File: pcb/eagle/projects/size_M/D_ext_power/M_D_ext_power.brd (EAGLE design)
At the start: 26 parts

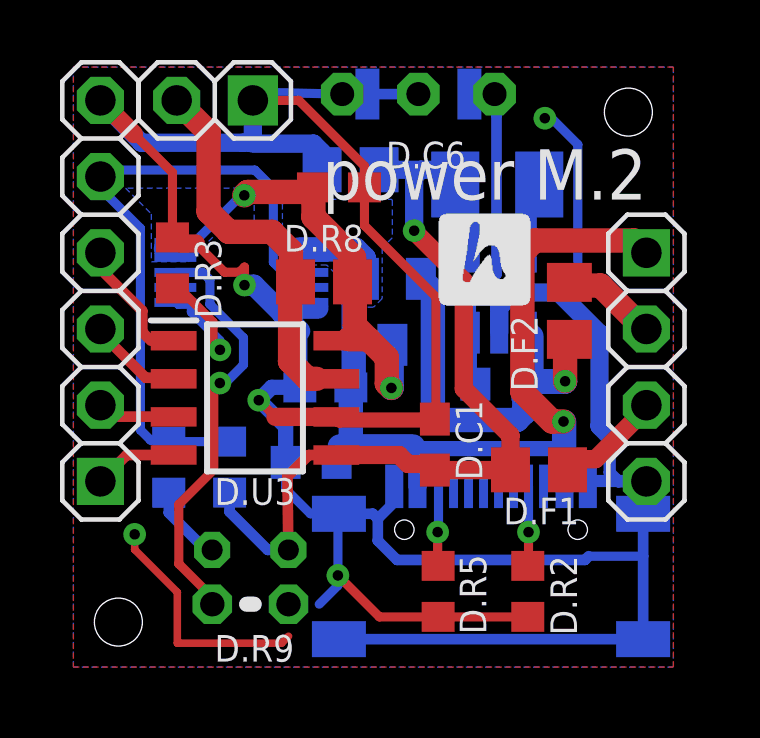
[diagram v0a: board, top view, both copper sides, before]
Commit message: closed PCB version M.2
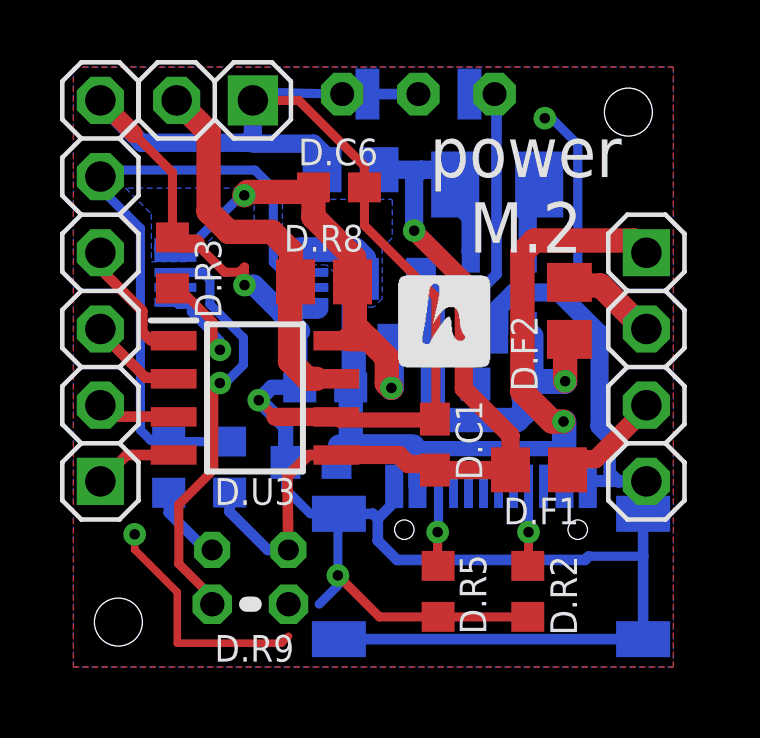
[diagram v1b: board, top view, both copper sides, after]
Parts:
- D.R6: value 2k2 -> 330
